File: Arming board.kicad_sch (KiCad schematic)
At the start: 14 parts, among them J1 Conn_01x04_Pin, J2 Conn_01x01_Pin, J3 Conn_01x01_Pin, Q1 SQS141ELNW-T1_GE3, Q2 SQS141ELNW-T1_GE3

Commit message: Add files via upload
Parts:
- D4: footprint (none) -> Diode_SMD:D_SOD-123
- F2: footprint (none) -> Fuse:Fuse_Bourns_TBU-CA
- J1: footprint (none) -> Connector_PinHeader_1.00mm:PinHeader_1x04_P1.00mm_Horizontal
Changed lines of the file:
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@@
 			)
 		)
-		(property "Footprint" ""
+		(property "Footprint" "Connector_PinHeader_1.00mm:PinHeader_1x04_P1.00mm_Horizontal"
 			(at 41.91 96.52 0)
 			(effects
@@
 			)
 		)
-		(property "Footprint" ""
+		(property "Footprint" "Fuse:Fuse_Bourns_TBU-CA"
 			(at 167.132 34.29 90)
 			(effects
@@
 			)
 		)
-		(property "Footprint" ""
+		(property "Footprint" "Diode_SMD:D_SOD-123"
 			(at 100.33 107.95 0)
 			(effects

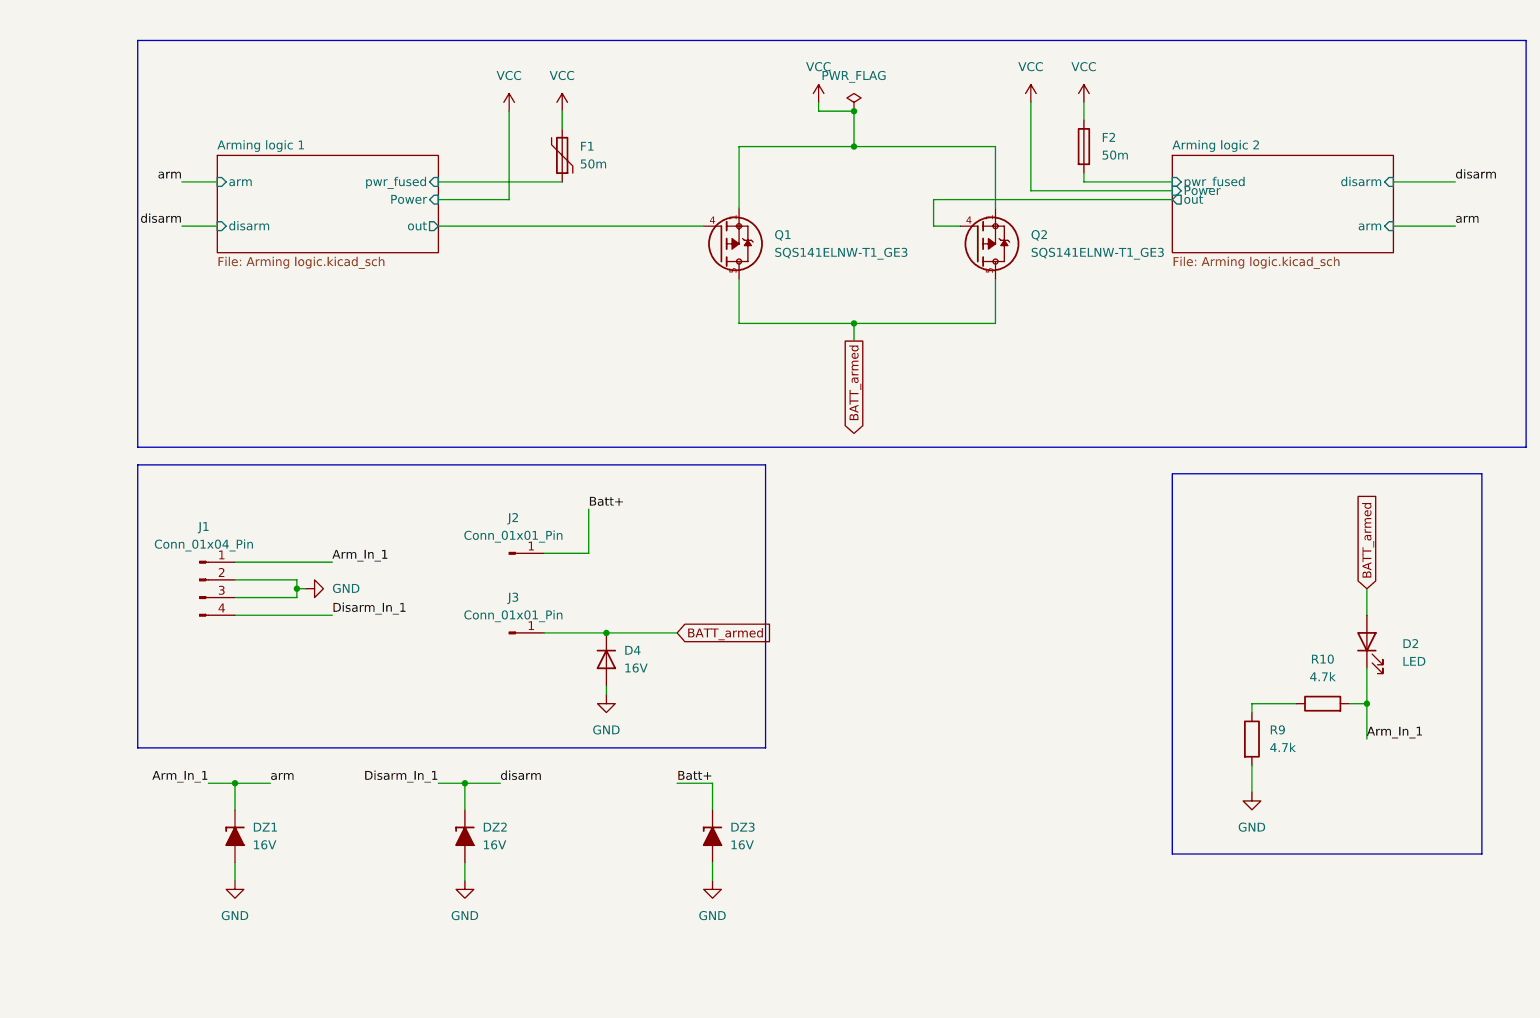
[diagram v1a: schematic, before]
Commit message: continued scematic
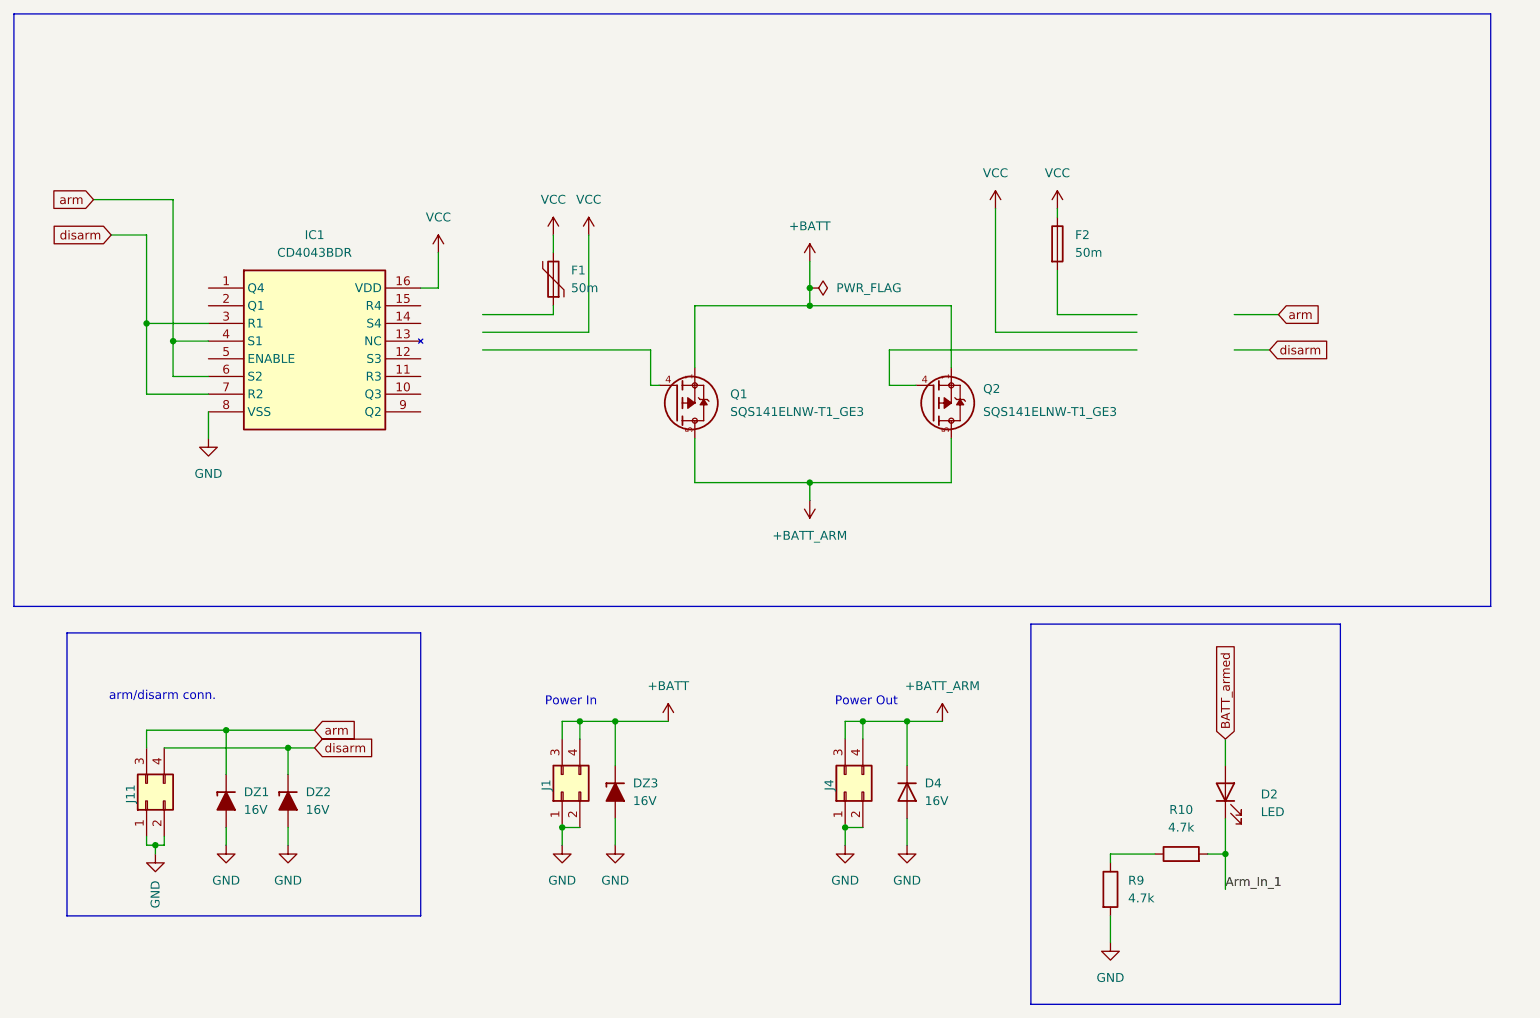
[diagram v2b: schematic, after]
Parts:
- removed J1: Conn_01x04_Pin, Connector_PinHeader_1.00mm:PinHeader_1x04_P1.00mm_Horizontal, symbol Connector:Conn_01x04_Pin
- removed J2, J3: Conn_01x01_Pin, Connector_PinHeader_1.00mm:PinHeader_1x01_P1.00mm_Horizontal, symbol Connector:Conn_01x01_Pin
- added IC1: CD4043BDR, SOIC127P600X175-16N, symbol rapid_arming:CD4043BDR
- added J1, J11, J4: ~, stigma:Molex_Micro-Fit_3.0_43045-0400_2x02_P3.00mm_Horizontal, symbol Connector_Generic:Conn_02x02_Top_Bottom
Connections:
- net Arm_In_1: no longer DZ1.1 (K)
- net BATT_armed: no longer D4.1 (K), Q1.5, Q1.6, Q1.7, Q1.8, Q1.9, Q2.5, Q2.6, Q2.7, Q2.8, Q2.9
- net GND: now also IC1.8 (VSS), J1.1 (Pin_1), J1.2 (Pin_2), J11.1 (Pin_1), J11.2 (Pin_2), J4.1 (Pin_1), J4.2 (Pin_2)
- net VCC: now also IC1.16 (VDD); no longer Q1.1, Q1.2, Q1.3, Q2.1, Q2.2, Q2.3
- net Arming logic 1/out: no longer names the net of Q1.4
- net Arming logic 1/pwr_fused: no longer names the net of F1.1
- net Arming logic 2/out: no longer names the net of Q2.4
- net Arming logic 2/pwr_fused: no longer names the net of F2.2
- net Batt+ renamed +BATT
- net +BATT: now also Q1.1, Q1.2, Q1.3, Q2.1, Q2.2, Q2.3, J1.3 (Pin_3), J1.4 (Pin_4)
- net Disarm_In_1 renamed disarm
- net disarm: now also IC1.3 (R1), IC1.7 (R2), J11.4 (Pin_4)
- new net +BATT_ARM: D4.1 (K), J4.3 (Pin_3), J4.4 (Pin_4), Q1.5, Q1.6, Q1.7, Q1.8, Q1.9, Q2.5, Q2.6, Q2.7, Q2.8, Q2.9
- new net arm: DZ1.1 (K), IC1.4 (S1), IC1.6 (S2), J11.3 (Pin_3)
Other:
- removed sheet Arming logic 1
- removed sheet Arming logic 2
- note added: "Power In"
- note added: "Power Out"
- note added: "arm/disarm conn."
- moved on the sheet: D2, D4, DZ1, DZ2, DZ3, F1, F2, Q1, Q2, R10, R9
